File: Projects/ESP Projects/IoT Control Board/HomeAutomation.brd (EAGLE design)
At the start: 73.6 x 98.7 mm, 37 parts, among them IC1 7805T, J1 OUT 1, J2 OUT 3, J3 OUT 4, J4 OUT 2, J5 POWER_JACK, K1 RELAY-SPDT-JZC-11F, K2 RELAY-SPDT-JZC-11F, K3 RELAY-SPDT-JZC-11F, K4 RELAY-SPDT-JZC-11F, T1 2N2222, T2 2N2222, T3 2N2222, T4 2N2222, U1 DHT22

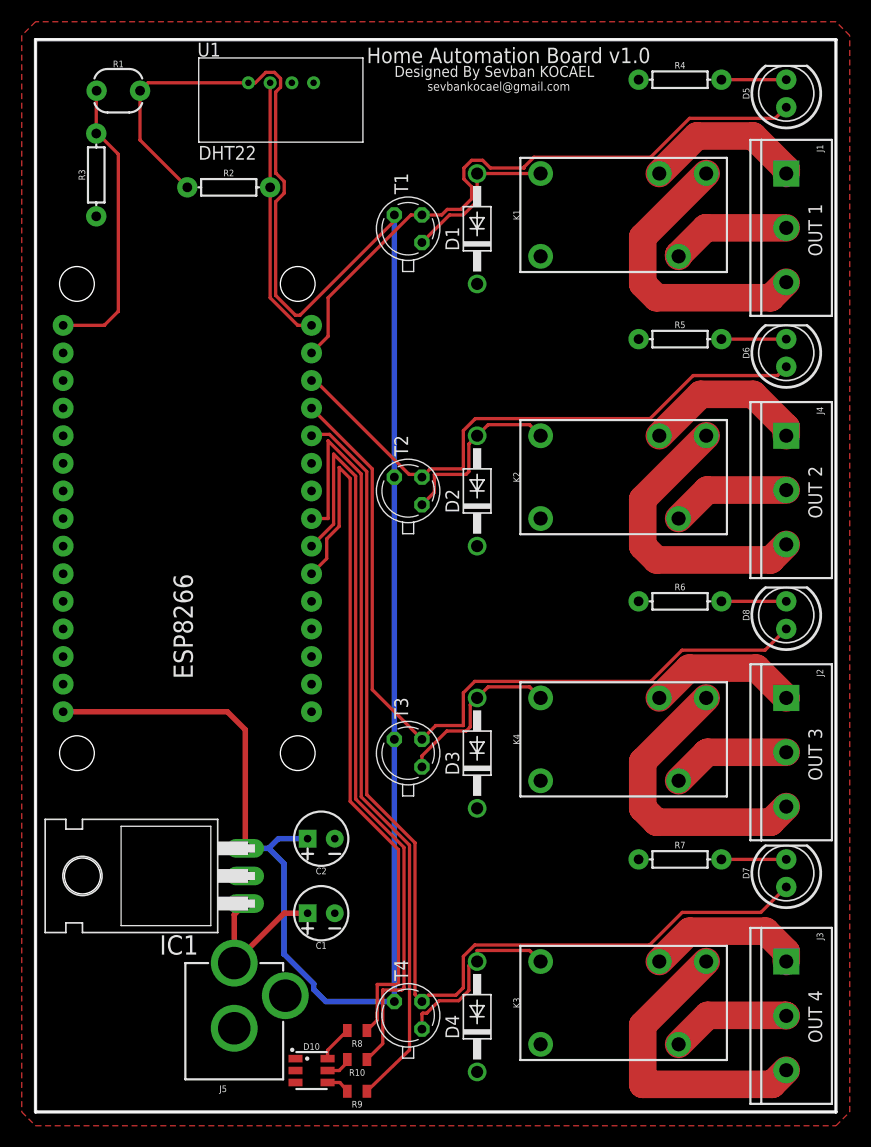
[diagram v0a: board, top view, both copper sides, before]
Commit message: Add files via upload
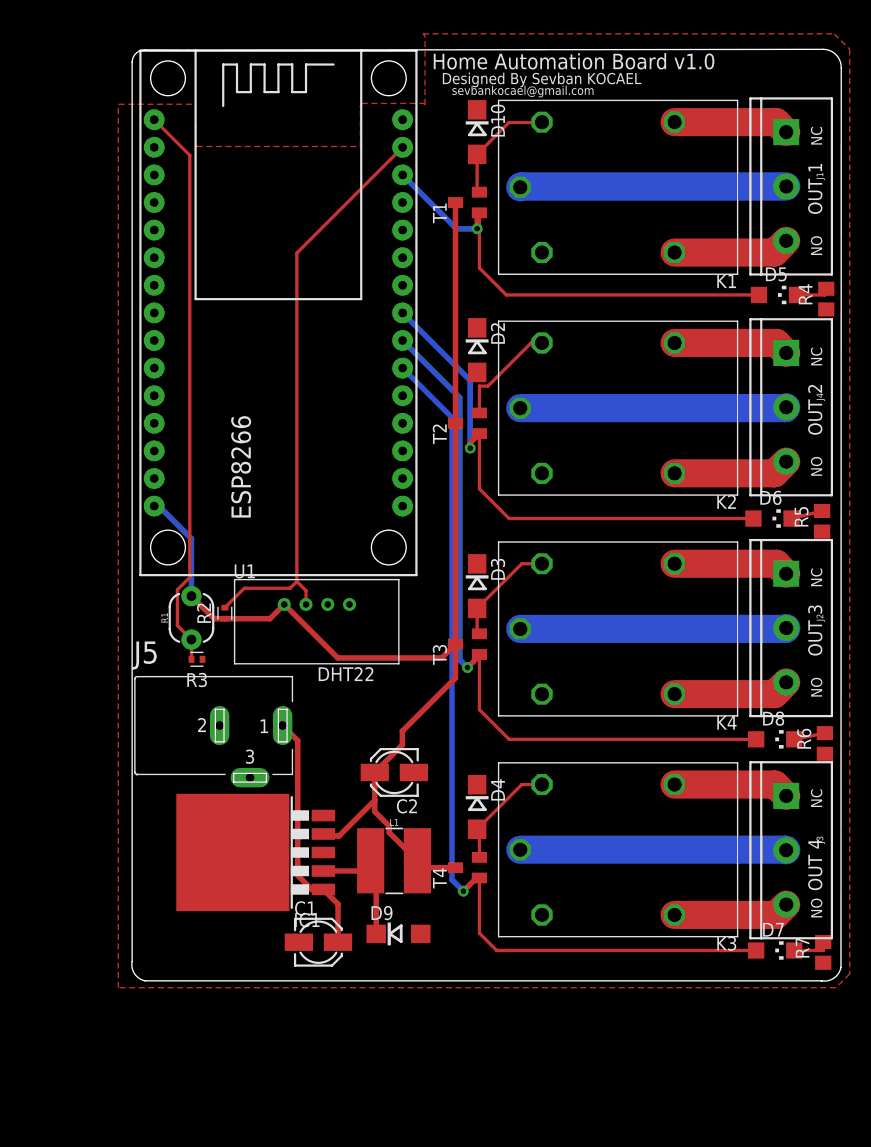
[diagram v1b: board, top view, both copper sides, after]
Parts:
- removed D1: 1N4004, diode:DO41-10
- removed R10, R8, R9: 0.3, SparkFun-Resistors:0805
- added D9: B340A-E3/61T, diode:DO214AC
- added L1: 33µH/±20%/1.4A, SparkFun-Coils:SRN6045
- C1: value 0.33uF -> 680uf; device SparkFun-Capacitors:CPOL-RADIAL-2.5MM-5MM-KIT -> rcl:153CLV-0405
- C2: value 0.1uF -> 220uF; device SparkFun-Capacitors:CPOL-RADIAL-2.5MM-5MM-KIT -> rcl:153CLV-0405
- D10: value RGB -> 1N4007; device SparkFun-LED:PLCC-6-LED -> diode:DO214AC
- D2, D3, D4: value 1N4004 -> 1N4007; device diode:DO41-10 -> diode:DO214AC
- D5, D6, D7, D8: device SparkFun-LED:LED_5MM -> led:CHIPLED_1206
- IC1: value 7805T -> LM2596S; device linear:TO220H -> national-semiconductor:TO263-5
- J5: value POWER_JACK -> 694106301002; device SparkFun-Connectors:POWER_JACK_PTH -> DC Power Jacks:694106301002
- K1, K2, K3, K4: value RELAY-SPDT-JZC-11F -> SIEMENS_V23082; device SparkFun-Electromechanical:RELAY-JZC -> LezzetliRobotTarifleri:SIEMENS_V23082_RELAY
- R2, R3: device SparkFun-Resistors:AXIAL-0.3 -> Resistor:RESC1005X40
- R4, R5, R6, R7: device SparkFun-Resistors:AXIAL-0.3 -> rcl:R0805
- T1, T2, T3, T4: device transistor:TO18 -> transistor:SOT23-BEC
- moved D10 87.7 mm to (127.0, 90.2), turned to 270 degrees
- moved R1 49.0 mm to (100.7, 45.5), turned to 90 degrees
- moved U1 48.1 mm to (111.3, 44.7)
- moved R3 45.5 mm to (101.2, 41.7), turned to 180 degrees
- moved R2 39.2 mm to (103.8, 45.9), turned to 90 degrees
- moved J5 36.7 mm to (95.5, 35.6)
- moved R4 24.3 mm to (159.1, 74.8), turned to 90 degrees
- moved R5 21.3 mm to (158.8, 54.4), turned to 90 degrees
- moved ESP8266 20.7 mm to (108.7, 73.5)
- moved D4 19.3 mm to (127.0, 28.1), turned to 270 degrees
- moved R6 18.7 mm to (159.0, 33.9), turned to 90 degrees
- moved D5 18.6 mm to (154.7, 75.2), turned to 270 degrees
- moved R7 15.7 mm to (158.9, 14.7), turned to 90 degrees
- moved D3 15.4 mm to (127.0, 48.4), turned to 270 degrees
- moved D6 15.3 mm to (154.2, 54.6), turned to 270 degrees
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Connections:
- removed net D0: ESP8266.D0, R2.P$2, U1.2
- removed net D3: D8.A, ESP8266.D3, T3.2
- removed net D4: D7.A, ESP8266.D4, T4.2
- removed net N$22: D10.AR, R10.2
- removed net N$24: D10.AG, R9.2
- removed net N$8: J3.1, K3.2
- new net N$26: D4.A, K3.P$1, T4.E
- net 5V: now also C2.+, IC1.4, L1.2, R2.1, T1.C, T2.C, T3.C, T4.C; no longer C2.1, IC1.3, R2.P$1, T1.3, T2.3, T3.3, T4.3
- net A0: now also R3.2; no longer R3.P$2
- net D1: now also R2.2, U1.2; no longer D5.A, T1.2
- net D2: now also D5.A, T1.B; no longer D6.A, T2.2
- net D5: now also D6.A, T2.B; no longer R9.1
- net D6: now also D8.A, T3.B; no longer R10.1
- net D7: now also D7.A, T4.B; no longer R8.1
- net GND: now also C1.-, C2.-, D10.C, D9.A, IC1.3, IC1.5, J5.2, J5.3, K1.P$2, K2.P$2, K3.P$2, K4.P$2, R3.1, R4.1, R5.1, R6.1, R7.1; no longer C1.2, C2.2, D1.C, D10.CB, D10.CG, D10.CR, IC1.2, J5.GND, J5.GNDBREAK, K1.1, K2.1, K3.1, K4.1, R3.P$1, R4.P$1, R5.P$1, R6.P$1, R7.P$1
- net N$1: now also D10.A, K1.P$1, T1.E; no longer D1.A, K1.5, T1.1
- net N$10: now also K3.P$4; no longer K3.3
- net N$11: now also K2.P$5; no longer K2.2
- net N$12: now also K2.P$3; no longer K2.4
- net N$13: now also K2.P$4; no longer K2.3
- net N$14: now also K1.P$4; no longer K1.3
- net N$15: now also K1.P$3; no longer K1.4
- net N$16: now also K1.P$5; no longer K1.2
- net N$17: now also D5.C, R4.2; no longer D5.K, R4.P$2
- net N$18: now also D6.C, R5.2; no longer D6.K, R5.P$2
- net N$19: now also C1.+, J5.1; no longer C1.1, J5.PWR
- net N$2: now also K4.P$5; no longer K4.2
- net N$20: now also D8.C, R6.2; no longer D8.K, R6.P$2
- net N$21: now also D7.C, R7.2; no longer D7.K, R7.P$2
- net N$23: now also D9.C, IC1.2, L1.1; no longer D10.AB, R8.2
- net N$3: now also K2.P$1, T2.E; no longer K2.5, T2.1
- net N$4: now also K4.P$3; no longer K4.4
- net N$5: now also K4.P$1, T3.E; no longer K4.5, T3.1
- net N$6: now also K4.P$4; no longer K4.3
- net N$7: now also J3.1, K3.P$5; no longer D4.A, K3.5, T4.1
- net N$9: now also K3.P$3; no longer K3.4
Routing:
- net D4: track 97.0 -> 0.00 mm
- net 5V: track 190.7 -> 113.4 mm
- net D3: track 74.2 -> 0.00 mm
- net D5: track 73.3 -> 48.1 mm, vias 0 -> 1
- net A0: track 26.9 -> 52.0 mm
- net D0: track 24.6 -> 0.00 mm
- net N$10: track 27.5 -> 10.7 mm
- net N$6: track 26.9 -> 10.7 mm
- net N$13: track 26.9 -> 10.7 mm
- net N$14: track 26.9 -> 10.7 mm
- net D7: track 67.5 -> 83.6 mm, vias 0 -> 1
- net N$8: track 14.5 -> 0.00 mm
- net N$12: track 11.0 -> 24.5 mm
- net N$4: track 11.0 -> 24.5 mm
- net N$9: track 11.0 -> 24.5 mm
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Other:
- board size 73.6 x 98.7 mm -> 65.3 x 85.7 mm
- board text added: "NC"
- board text added: "NO"
